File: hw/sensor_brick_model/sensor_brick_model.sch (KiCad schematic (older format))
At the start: 13 parts, among them J1 Conn_01x04_Male, J2 Conn_01x06_Male, U1 BMI160

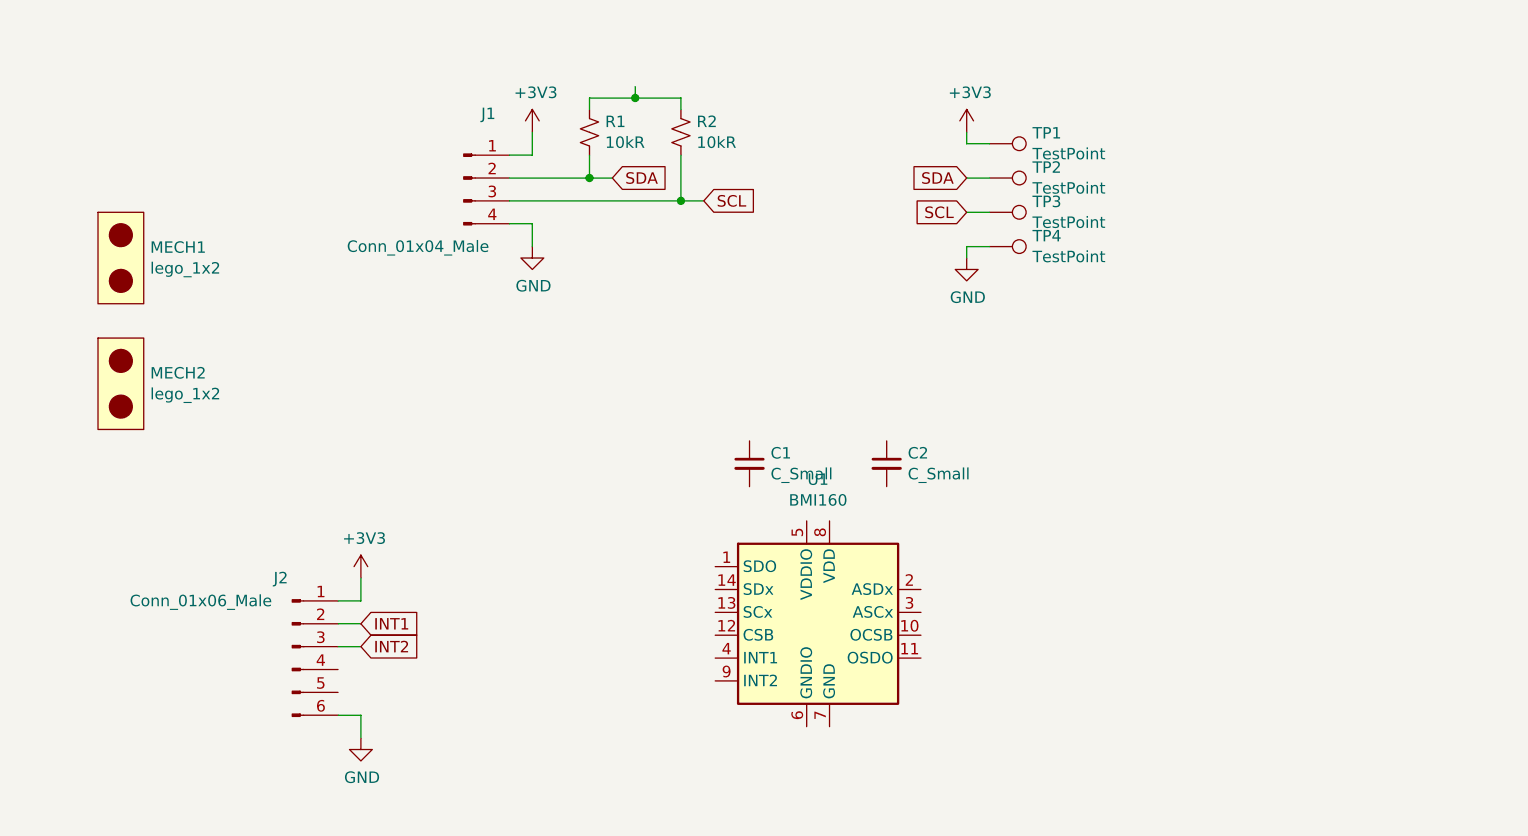
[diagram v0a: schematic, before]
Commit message: Version 1A done
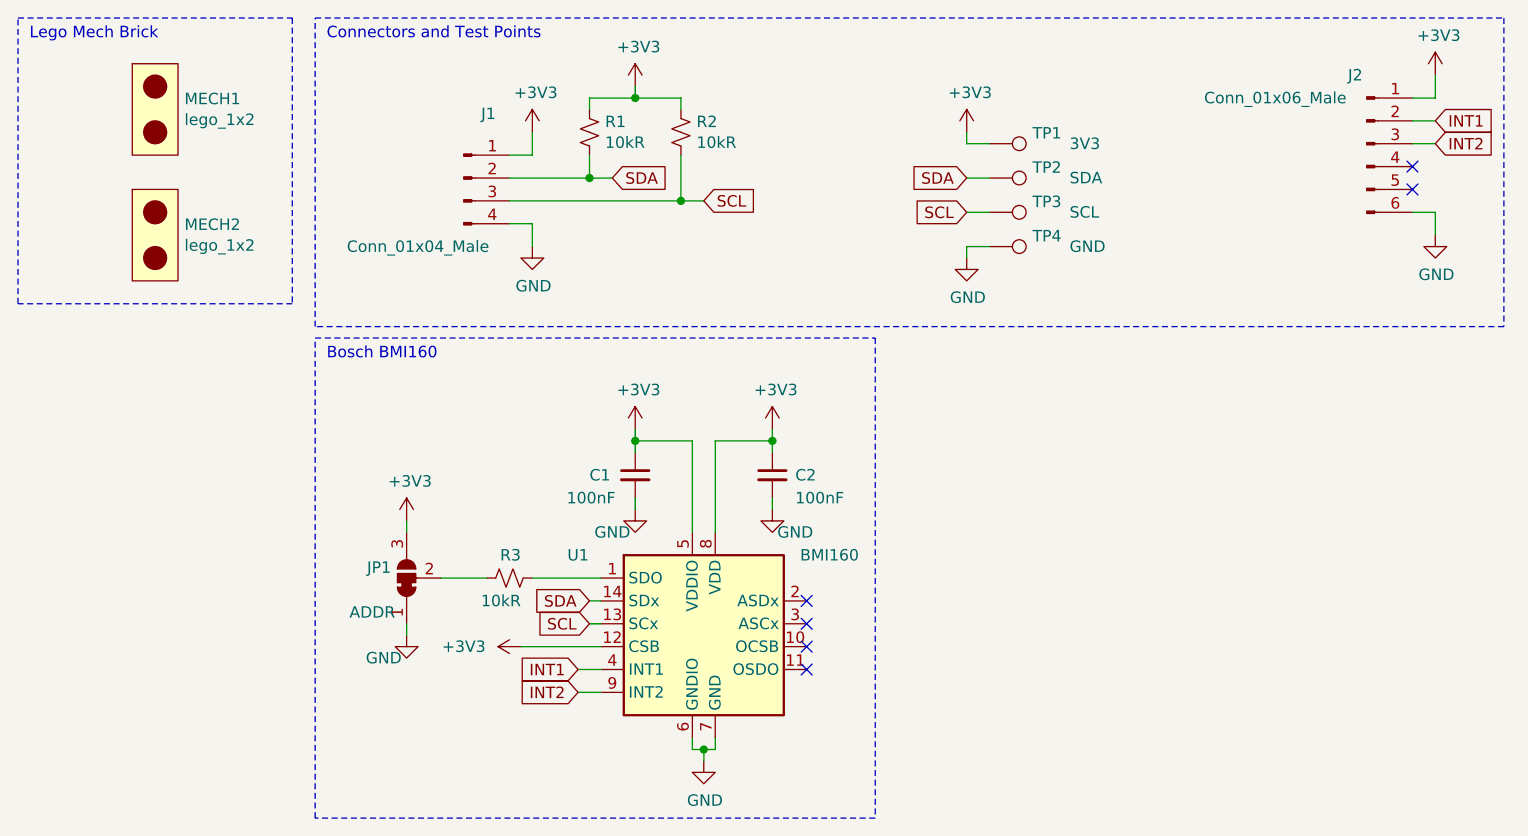
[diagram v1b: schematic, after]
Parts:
- added JP1: ADDR, Jumper:SolderJumper-3_P1.3mm_Bridged12_RoundedPad1.0x1.5mm, symbol Jumper:SolderJumper_3_Bridged12
- added R3: 10kR, Resistor_SMD:R_0603_1608Metric, symbol Device:R_Small_US
- C1, C2: value C_Small -> 100nF; footprint Capacitor_SMD:C_0402_1005Metric -> Capacitor_SMD:C_0603_1608Metric
- R1, R2: footprint Resistor_SMD:R_0402_1005Metric -> Resistor_SMD:R_0603_1608Metric
- TP1: value TestPoint -> 3V3
- TP2: value TestPoint -> SDA
- TP3: value TestPoint -> SCL
- TP4: value TestPoint -> GND
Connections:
- wire segments 27 -> 51
- no-connect marks 0 -> 6
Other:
- note added: "Bosch BMI160"
- note added: "Connectors and Test Points"
- note added: "Lego Mech Brick"
- moved on the sheet: C1, C2, J2, MECH1, MECH2, U1
